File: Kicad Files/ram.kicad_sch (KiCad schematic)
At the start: 20 parts, among them U13 HM62256BLP, U14 74LS245

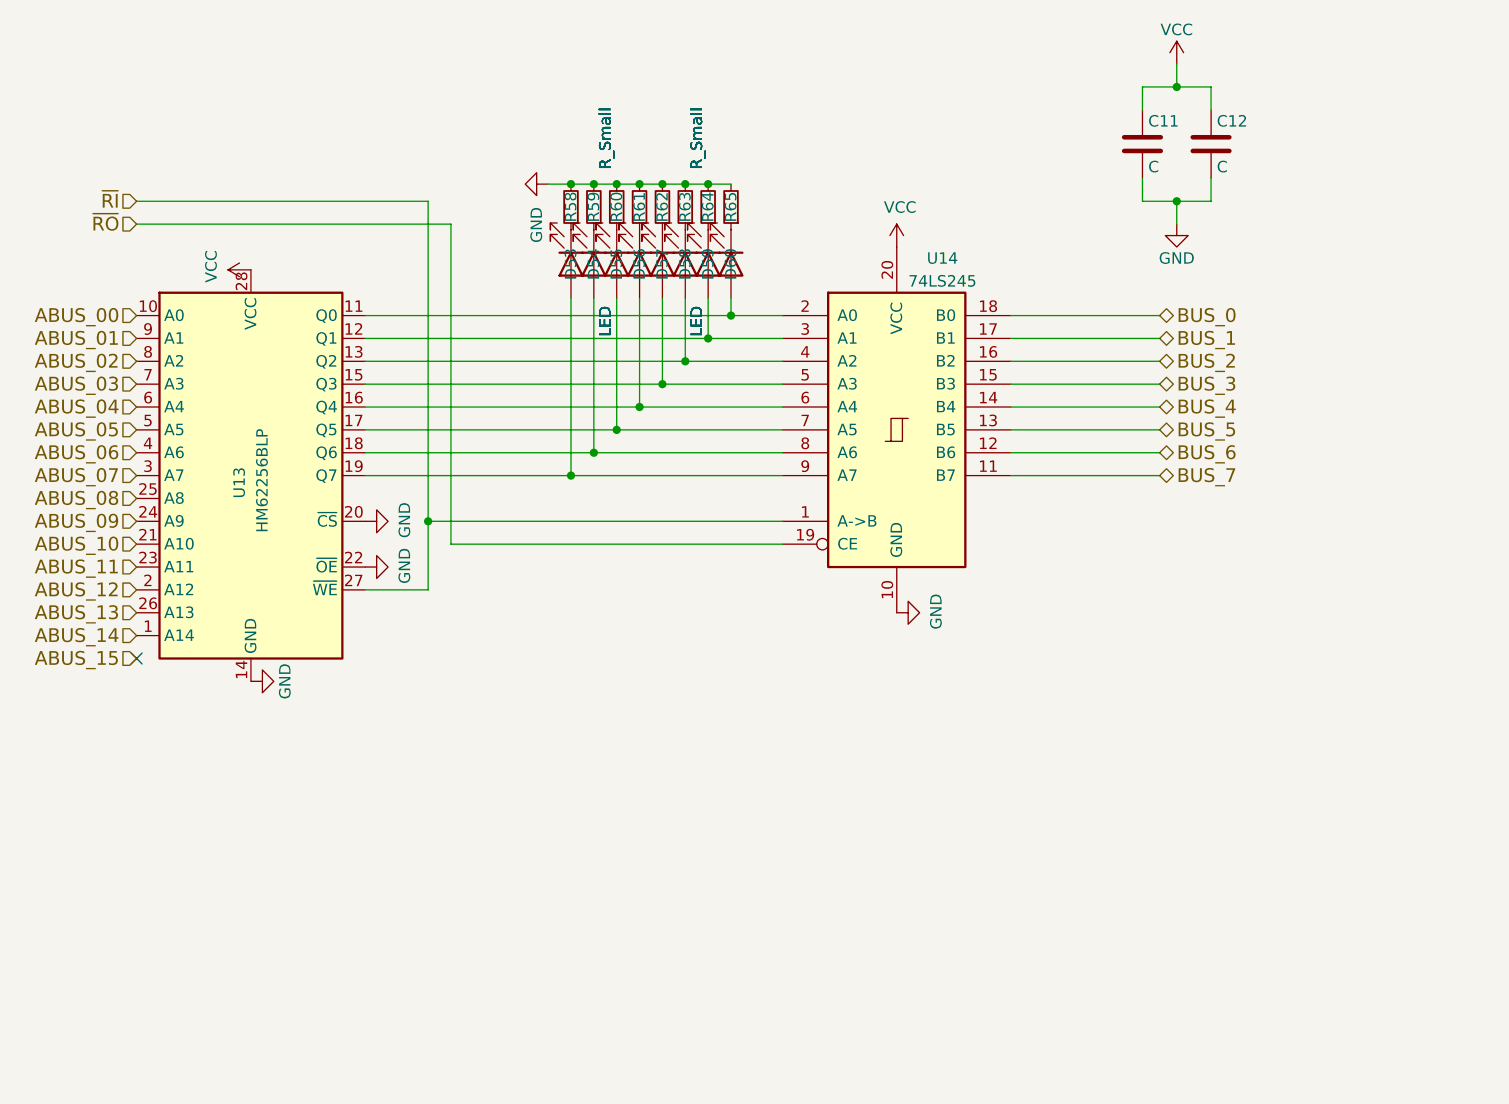
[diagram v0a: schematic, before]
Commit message: np2
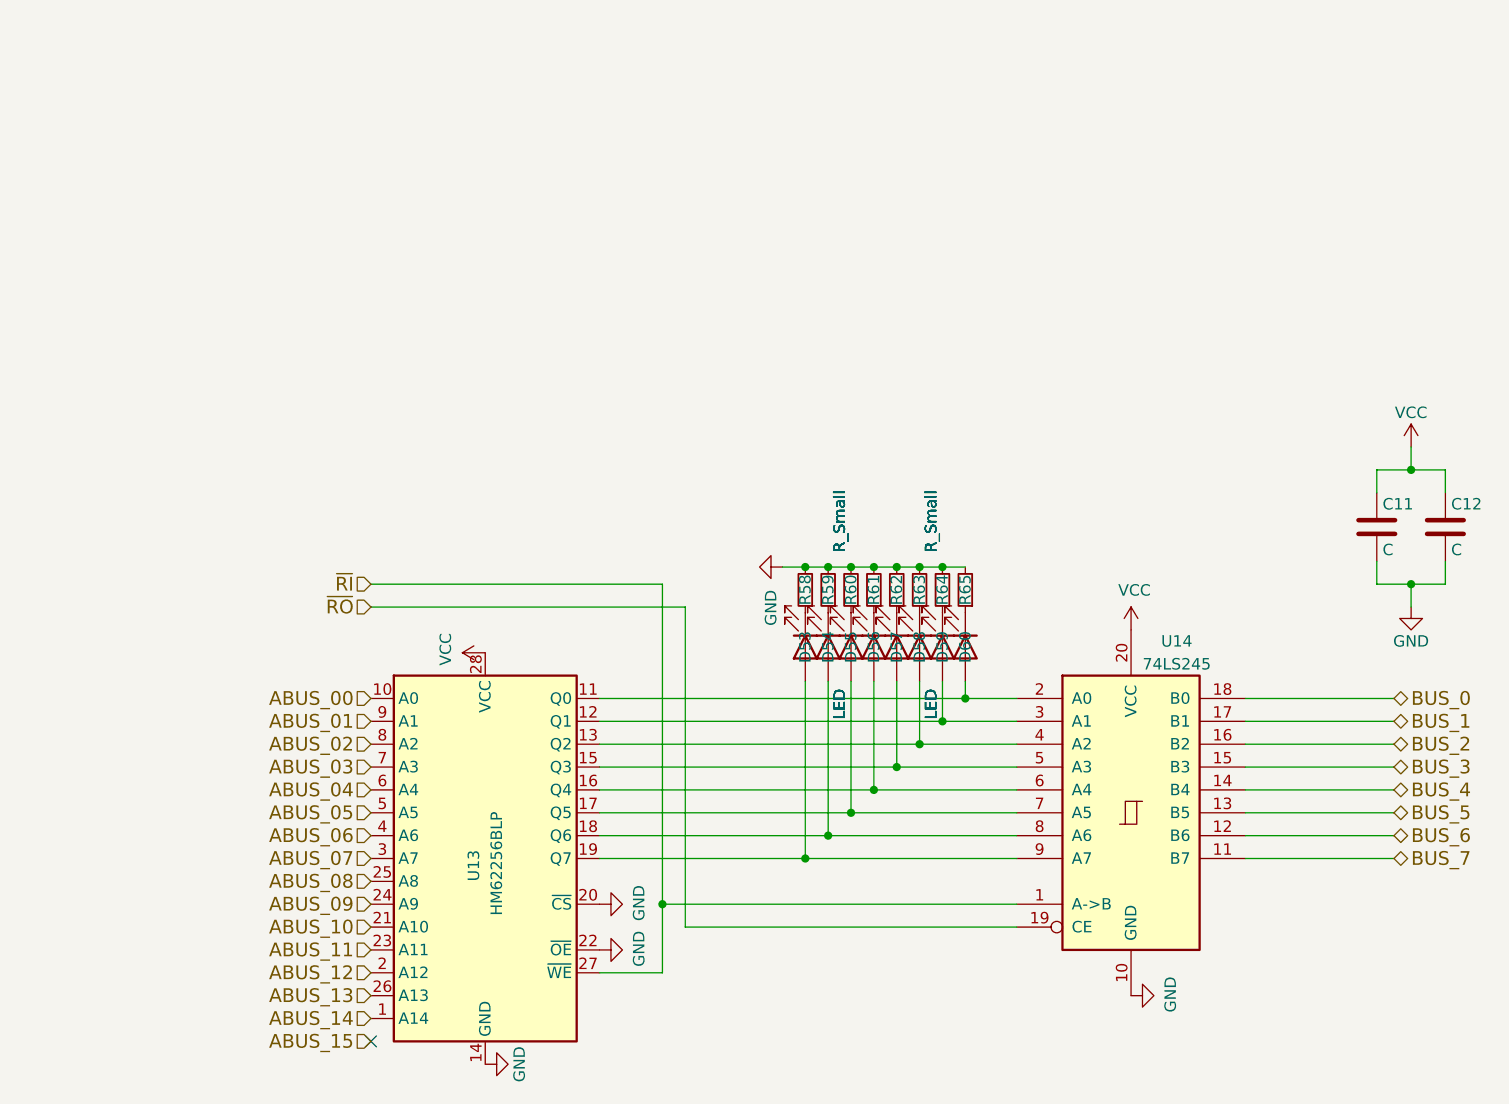
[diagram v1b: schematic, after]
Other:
- moved on the sheet: C11, C12, D53, D54, D55, D56, D57, D58, D59, D60, R58, R59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
